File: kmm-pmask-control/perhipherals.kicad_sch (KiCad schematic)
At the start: 2 parts, among them J4 0472192001, J5 Conn_ARM_JTAG_SWD_10

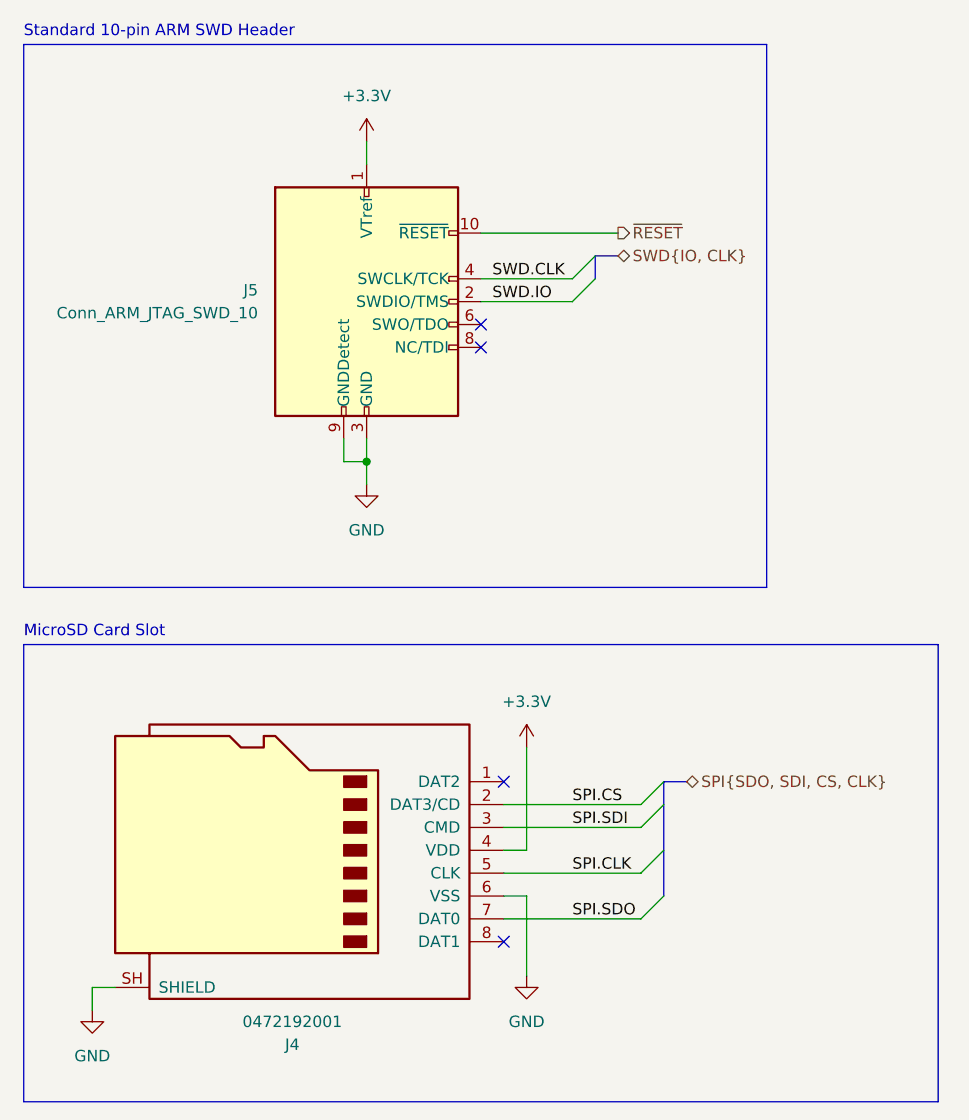
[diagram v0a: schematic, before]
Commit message: Initial PCB Layout
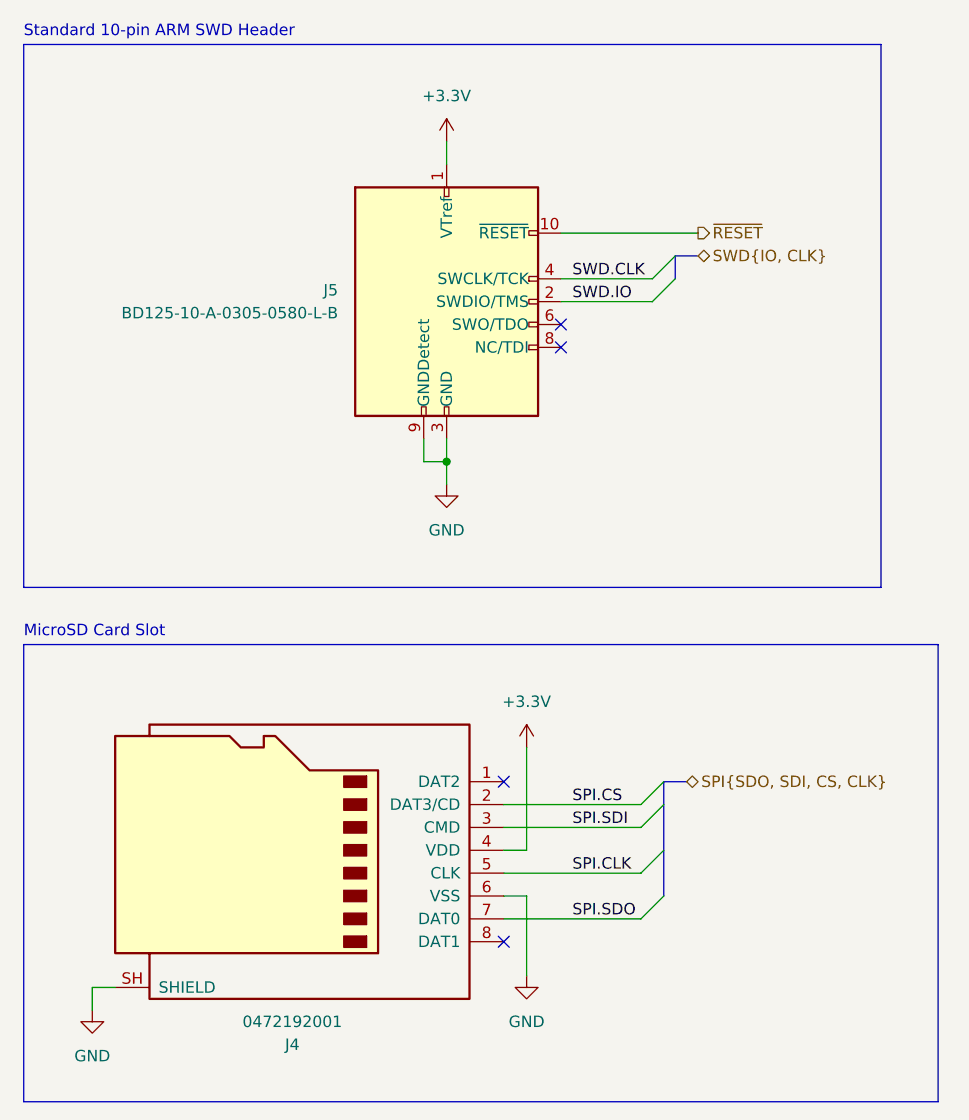
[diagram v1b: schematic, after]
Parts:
- J5: value Conn_ARM_JTAG_SWD_10 -> BD125-10-A-0305-0580-L-B; Manufacturer P/N (none) -> BD125-10-A-0305-0580-L-B; Vendor (none) -> DigiKey; Vendor P/N (none) -> 2073-BD125-10-A-0305-0580-L-BCT-ND
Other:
- moved on the sheet: J5
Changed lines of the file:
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@@
 	(rectangle
 		(start 88.9 38.735)
-		(end 171.45 99.06)
+		(end 184.15 99.06)
 		(stroke
 			(width 0)
@@
 	)
 	(junction
-		(at 127 85.09)
+		(at 135.89 85.09)
 		(diameter 0)
 		(color 0 0 0 0)
 	)
 	(no_connect
-		(at 139.7 72.39)
+		(at 148.59 72.39)
 	)
 	(no_connect
@@
 	)
 	(no_connect
-		(at 139.7 69.85)
+		(at 148.59 69.85)
 	)
 	(bus_entry
@@
 	)
 	(bus_entry
-		(at 149.86 64.77)
+		(at 158.75 64.77)
 		(size 2.54 -2.54)
 		(stroke
@@
 	)
 	(bus_entry
-		(at 149.86 67.31)
+		(at 158.75 67.31)
 		(size 2.54 -2.54)
 		(stroke
@@
 	(wire
 		(pts
-			(xy 127 87.63) (xy 127 85.09)
+			(xy 135.89 87.63) (xy 135.89 85.09)
 		)
 		(stroke
@@
 	(wire
 		(pts
-			(xy 139.7 59.69) (xy 154.94 59.69)
-		)
-		(stroke
-			(width 0)
-			(type default)
-		)
-	)
-	(wire
-		(pts
-			(xy 124.46 82.55) (xy 124.46 85.09)
-		)
-		(stroke
-			(width 0)
-			(type default)
-		)
-	)
-	(wire
-		(pts
-			(xy 124.46 85.09) (xy 127 85.09)
-		)
-		(stroke
-			(width 0)
-			(type default)
-		)
-	)
-	(wire
-		(pts
-			(xy 139.7 67.31) (xy 149.86 67.31)
+			(xy 148.59 59.69) (xy 163.83 59.69)
+		)
+		(stroke
+			(width 0)
+			(type default)
+		)
+	)
+	(wire
+		(pts
+			(xy 133.35 82.55) (xy 133.35 85.09)
+		)
+		(stroke
+			(width 0)
+			(type default)
+		)
+	)
+	(wire
+		(pts
+			(xy 133.35 85.09) (xy 135.89 85.09)
+		)
+		(stroke
+			(width 0)
+			(type default)
+		)
+	)
+	(wire
+		(pts
+			(xy 148.59 67.31) (xy 158.75 67.31)
 		)
 		(stroke
@@
 	(wire
 		(pts
-			(xy 139.7 64.77) (xy 149.86 64.77)
+			(xy 148.59 64.77) (xy 158.75 64.77)
 		)
 		(stroke
@@
 	(bus
 		(pts
-			(xy 152.4 62.23) (xy 154.94 62.23)
+			(xy 161.29 62.23) (xy 163.83 62.23)
 		)
 		(stroke
@@
 	(wire
 		(pts
-			(xy 127 82.55) (xy 127 85.09)
+			(xy 135.89 82.55) (xy 135.89 85.09)
 		)
 		(stroke
@@
 	(wire
 		(pts
-			(xy 127 49.53) (xy 127 52.07)
+			(xy 135.89 49.53) (xy 135.89 52.07)
 		)
 		(stroke
@@
 	(bus
 		(pts
-			(xy 152.4 64.77) (xy 152.4 62.23)
+			(xy 161.29 64.77) (xy 161.29 62.23)
 		)
 		(stroke
@@
 	)
 	(label "SWD.CLK"
-		(at 140.97 64.77 0)
+		(at 149.86 64.77 0)
 		(effects
 			(font
@@
 	)
 	(label "SWD.IO"
-		(at 140.97 67.31 0)
+		(at 149.86 67.31 0)
 		(effects
 			(font
@@
 	(hierarchical_label "~{RESET}"
 		(shape output)
-		(at 154.94 59.69 0)
+		(at 163.83 59.69 0)
 		(effects
 			(font
@@
 	(hierarchical_label "SWD{IO, CLK}"
 		(shape bidirectional)
-		(at 154.94 62.23 0)
+		(at 163.83 62.23 0)
 		(effects
 			(font
@@
 	(symbol
 		(lib_id "power:GND")
-		(at 127 87.63 0)
+		(at 135.89 87.63 0)
 		(unit 1)
 		(body_style 1)
@@
 		(fields_autoplaced yes)
 		(property "Reference" "#PWR034"
-			(at 127 93.98 0)
+			(at 135.89 93.98 0)
 			(hide yes)
 			(show_name no)
@@
 		)
 		(property "Value" "GND"
-			(at 127 92.71 0)
+			(at 135.89 92.71 0)
 			(show_name no)
 			(do_not_autoplace no)
@@
 		)
 		(property "Footprint" ""
-			(at 127 87.63 0)
+			(at 135.89 87.63 0)
 			(hide yes)
 			(show_name no)
@@
 		)
 		(property "Datasheet" ""
-			(at 127 87.63 0)
+			(at 135.89 87.63 0)
 			(hide yes)
 			(show_name no)
@@
 		)
 		(property "Description" "Power symbol creates a global label with name \"GND\" , ground"
-			(at 127 87.63 0)
+			(at 135.89 87.63 0)
 			(hide yes)
 			(show_name no)
@@
 	(symbol
 		(lib_id "power:+3.3V")
-		(at 127 49.53 0)
+		(at 135.89 49.53 0)
 		(unit 1)
 		(body_style 1)
@@
 		(fields_autoplaced yes)
 		(property "Reference" "#PWR033"
-			(at 127 53.34 0)
+			(at 135.89 53.34 0)
 			(hide yes)
 			(show_name no)
@@
 		)
 		(property "Value" "+3.3V"
-			(at 127 44.45 0)
+			(at 135.89 44.45 0)
 			(show_name no)
 			(do_not_autoplace no)
@@
 		)
 		(property "Footprint" ""
-			(at 127 49.53 0)
+			(at 135.89 49.53 0)
 			(hide yes)
 			(show_name no)
@@
 		)
 		(property "Datasheet" ""
-			(at 127 49.53 0)
+			(at 135.89 49.53 0)
 			(hide yes)
 			(show_name no)
@@
 		)
 		(property "Description" "Power symbol creates a global label with name \"+3.3V\""
-			(at 127 49.53 0)
+			(at 135.89 49.53 0)
 			(hide yes)
 			(show_name no)
@@
 	(symbol
 		(lib_id "Connector:Conn_ARM_JTAG_SWD_10")
-		(at 127 67.31 0)
+		(at 135.89 67.31 0)
 		(unit 1)
 		(body_style 1)
@@
 		(fields_autoplaced yes)
 		(property "Reference" "J5"
-			(at 114.935 66.0399 0)
+			(at 123.825 66.0399 0)
 			(show_name no)
 			(do_not_autoplace no)
@@
 			)
 		)
-		(property "Value" "Conn_ARM_JTAG_SWD_10"
-			(at 114.935 68.5799 0)
+		(property "Value" "BD125-10-A-0305-0580-L-B"
+			(at 123.825 68.5799 0)
 			(show_name no)
 			(do_not_autoplace no)
@@
 		)
 		(property "Footprint" "Connector_PinHeader_1.27mm:PinHeader_2x05_P1.27mm_Vertical_SMD"
-			(at 127 67.31 0)
+			(at 135.89 67.31 0)
 			(hide yes)
 			(show_name no)
@@
 		)
 		(property "Datasheet" "http://infocenter.arm.com/help/topic/com.arm.doc.ddi0314h/DDI0314H_coresight_components_trm.pdf"
-			(at 118.11 99.06 90)
+			(at 127 99.06 90)
 			(hide yes)
 			(show_name no)
@@
 		)
 		(property "Description" "Cortex Debug Connector, standard ARM Cortex-M SWD and JTAG interface"
-			(at 127 67.31 0)
-			(hide yes)
-			(show_name no)
+			(at 135.89 67.31 0)
+			(hide yes)
+			(show_name no)
+			(do_not_autoplace no)
+			(effects
+				(font
+					(size 1.27 1.27)
+				)
+			)
+		)
+		(property "Manufacturer P/N" "BD125-10-A-0305-0580-L-B"
+			(at 135.89 67.31 0)
+			(hide yes)
+			(show_name no)
+			(do_not_autoplace no)
+			(effects
+				(font
+					(size 1.27 1.27)
+				)
+			)
+		)
+		(property "Vendor" "DigiKey"
+			(at 135.89 67.31 0)
+			(hide yes)
+			(show_name no)
+			(do_not_autoplace no)
+			(effects
+				(font
+					(size 1.27 1.27)
+				)
+			)
+		)
+		(property "Vendor P/N" "2073-BD125-10-A-0305-0580-L-BCT-ND"
+			(at 135.89 67.31 0)
+			(hide yes)
+			(show_name no)
